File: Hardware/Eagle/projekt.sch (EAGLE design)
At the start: 134 parts, among them IC1 MEGA16-P, Q1 BC807-40SMD, Q10 2N2222, Q11 2N2222, Q12 2N2222, Q13 BC807-40SMD, Q14 BC807-40SMD, Q15 BC807-40SMD, Q16 BC807-40SMD, Q17 BC807-40SMD, Q18 BC807-40SMD, Q19 BC807-40SMD, Q2 BC807-40SMD, Q20 2N2222, Q22 2N2222, Q24 2N2222, Q26 2N2222, Q27 2N2222, Q29 2N2222, Q3 BC807-40SMD, Q30 2N2222, Q4 BC807-40SMD, Q5 BC807-40SMD, Q6 2N2222, Q7 2N2222, Q8 2N2222, Q9 2N2222

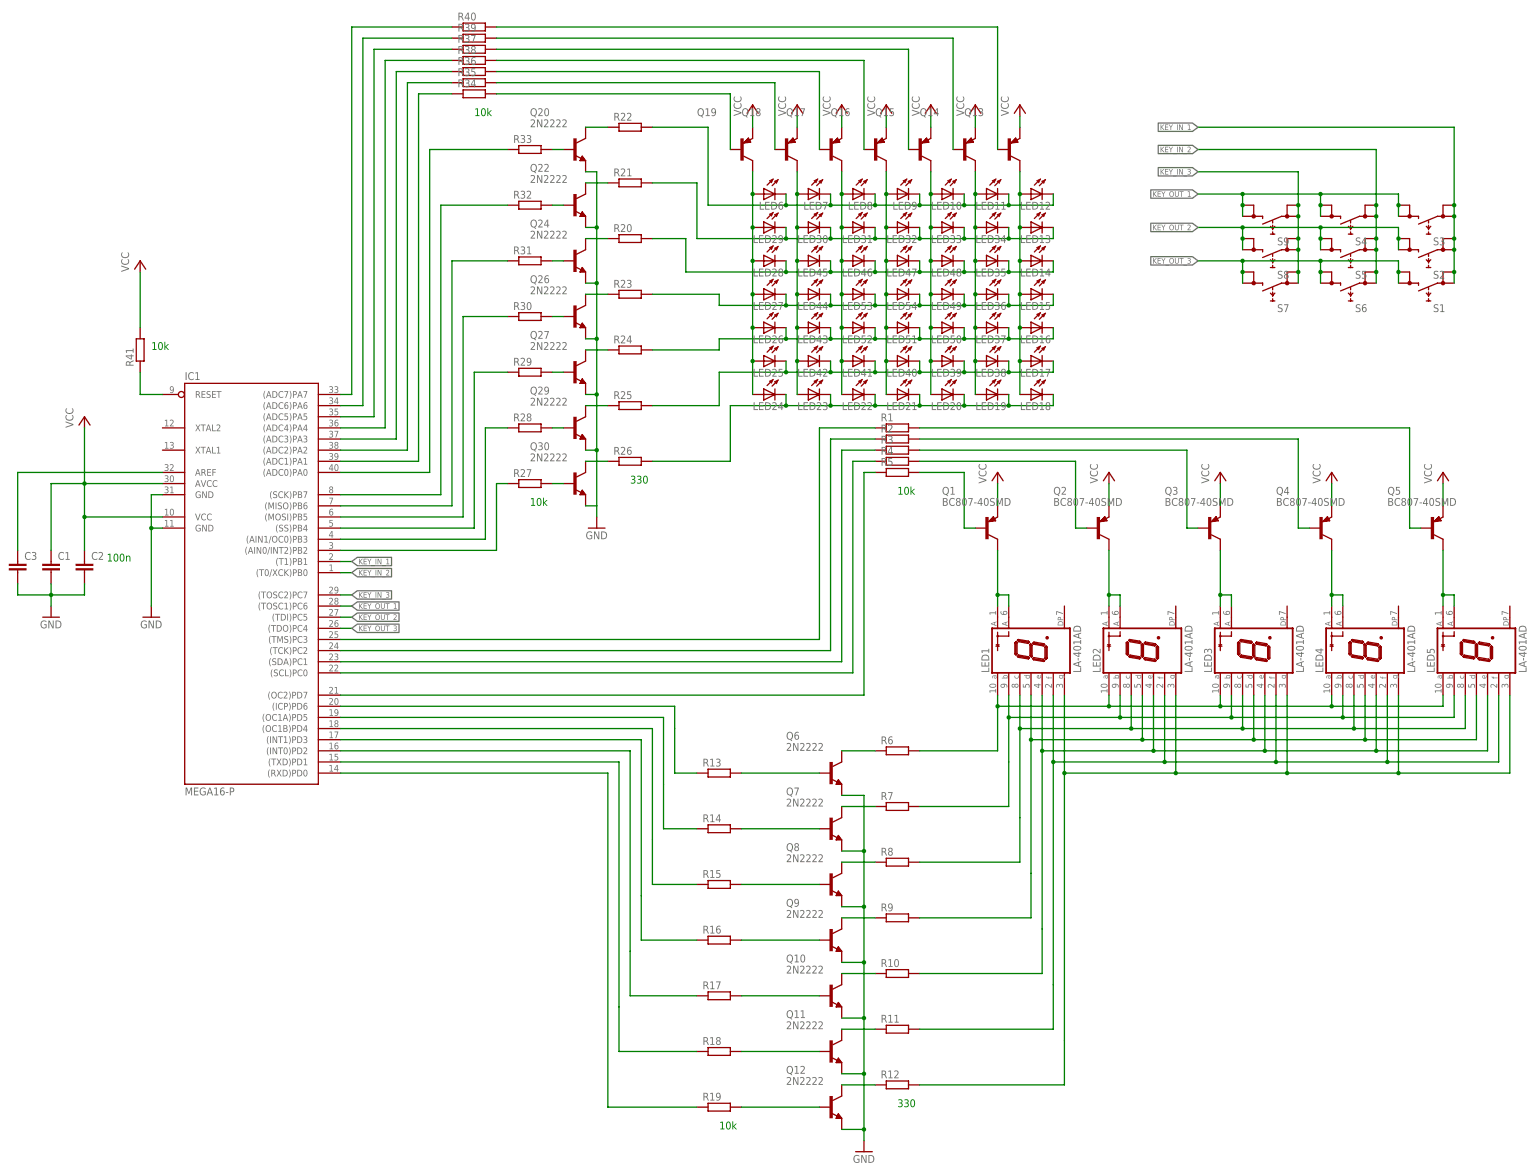
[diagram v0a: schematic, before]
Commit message: pierwsza wersja zasilania
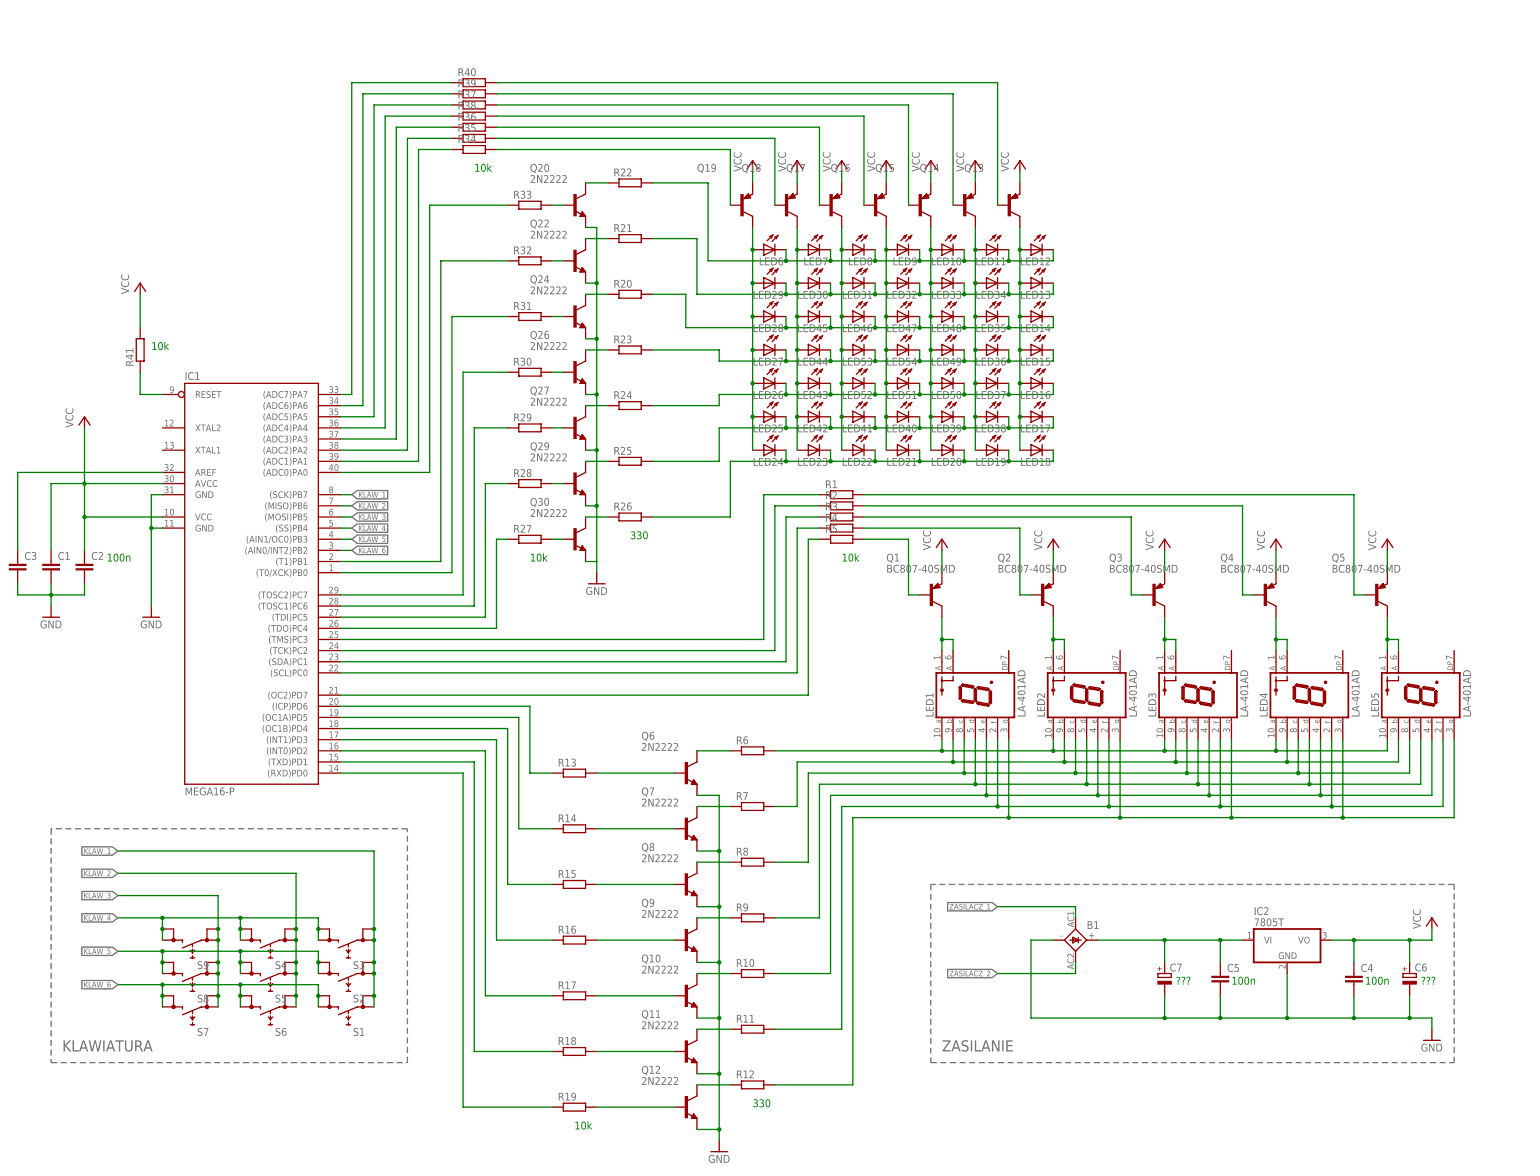
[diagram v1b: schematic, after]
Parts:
- added B1: (no value), rectifier:KBU
- added C4, C5: (no value), capacitor-wima:C5/7.2
- added C6, C7: (no value), rcl:CPOL-EUB45181C
- added IC2: 7805T, linear:7805T
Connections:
- removed net KEY_IN_1: IC1.(T1)PB1, S1.0@A, S1.0@B, S2.0@A, S2.0@B, S3.0@A, S3.0@B
- removed net KEY_IN_2: IC1.(T0/XCK)PB0, S4.0@A, S4.0@B, S5.0@A, S5.0@B, S6.0@A, S6.0@B
- removed net KEY_IN_3: IC1.(TOSC2)PC7, S7.0@A, S7.0@B, S8.0@A, S8.0@B, S9.0@A, S9.0@B
- removed net KEY_OUT_1: IC1.(TOSC1)PC6, S3.1@A, S3.1@B, S4.1@A, S4.1@B, S9.1@A, S9.1@B
- removed net KEY_OUT_2: IC1.(TDI)PC5, S2.1@A, S2.1@B, S5.1@A, S5.1@B, S8.1@A, S8.1@B
- removed net KEY_OUT_3: IC1.(TDO)PC4, S1.1@A, S1.1@B, S6.1@A, S6.1@B, S7.1@A, S7.1@B
- new net KLAW_1: IC1.(SCK)PB7, S1.0@A, S1.0@B, S2.0@A, S2.0@B, S3.0@A, S3.0@B
- new net KLAW_2: IC1.(MISO)PB6, S4.0@A, S4.0@B, S5.0@A, S5.0@B, S6.0@A, S6.0@B
- new net KLAW_3: IC1.(MOSI)PB5, S7.0@A, S7.0@B, S8.0@A, S8.0@B, S9.0@A, S9.0@B
- new net KLAW_4: IC1.(SS)PB4, S3.1@A, S3.1@B, S4.1@A, S4.1@B, S9.1@A, S9.1@B
- new net KLAW_5: IC1.(AIN1/OC0)PB3, S2.1@A, S2.1@B, S5.1@A, S5.1@B, S8.1@A, S8.1@B
- new net KLAW_6: IC1.(AIN0/INT2)PB2, S1.1@A, S1.1@B, S6.1@A, S6.1@B, S7.1@A, S7.1@B
- new net N$26: B1.+, C5.1, C7.+, IC2.VI
- new net ZASILACZ_1: B1.AC1
- new net ZASILACZ_2: B1.AC2
- net GND: now also B1.-, C4.2, C5.2, C6.-, C7.-, IC2.GND
- net N$50: now also IC1.(TDO)PC4; no longer IC1.(AIN0/INT2)PB2
- net N$64: now also IC1.(TDI)PC5; no longer IC1.(AIN1/OC0)PB3
- net N$67: now also IC1.(TOSC1)PC6; no longer IC1.(SS)PB4
- net N$68: now also IC1.(TOSC2)PC7; no longer IC1.(MOSI)PB5
- net N$69: now also IC1.(T0/XCK)PB0; no longer IC1.(MISO)PB6
- net N$70: now also IC1.(T1)PB1; no longer IC1.(SCK)PB7
- net VCC: now also C4.1, C6.+, IC2.VO
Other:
- note added: "???"
- note added: "KLAWIATURA"
- note added: "ZASILANIE"
- moved on the sheet: LED1, LED10, LED11, LED12, LED13, LED14, LED15, LED16, LED17, LED18, LED19, LED2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
